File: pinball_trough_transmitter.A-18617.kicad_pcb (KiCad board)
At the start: 2 copper layers, 162.6 x 88.5 mm, 16 parts, among them J1 Conn_01x09_Male, J2 Conn_01x09_Male, Q1 SFH460, Q2 SFH460, Q3 SFH460, Q4 SFH460, Q5 SFH460, Q6 SFH460, Q7 SFH460

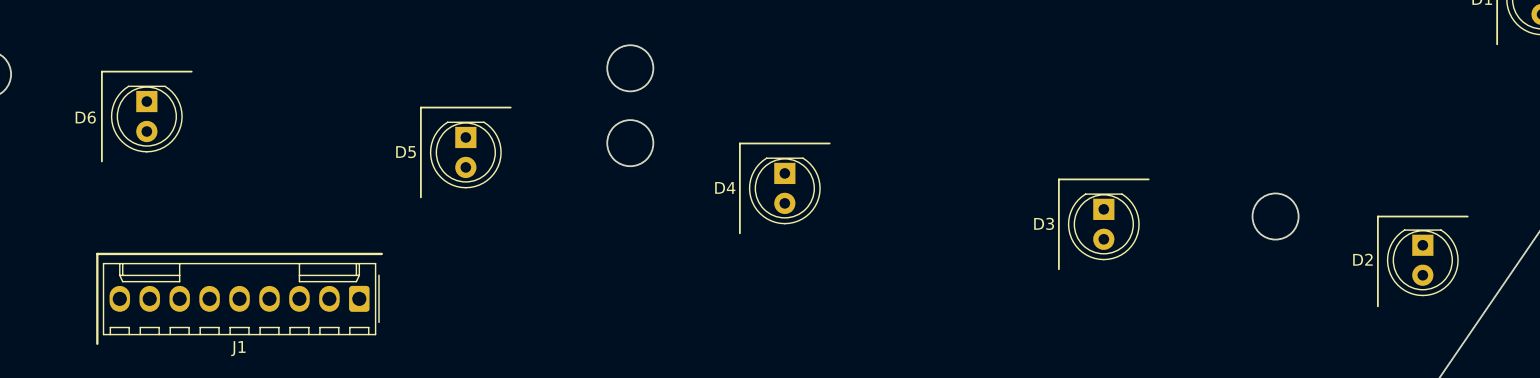
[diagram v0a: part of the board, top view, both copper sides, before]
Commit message: Minor adjustments
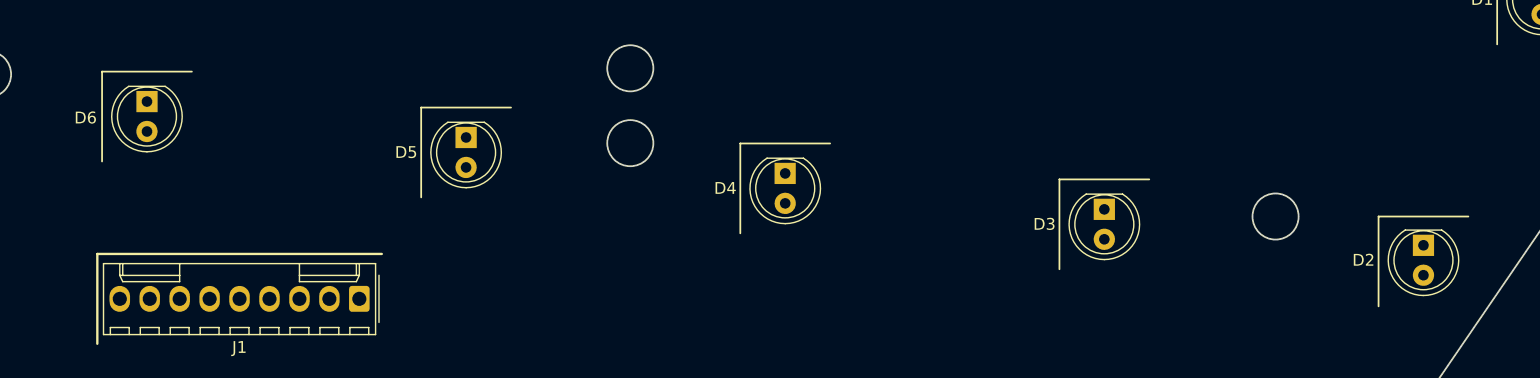
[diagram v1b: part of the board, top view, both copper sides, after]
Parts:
- moved D2 0.06 mm to (212.2, 72.3)
